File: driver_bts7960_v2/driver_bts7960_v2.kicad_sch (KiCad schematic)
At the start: 28 parts, among them J1 Motor_1, J2 Alimentacion, J6 Motor_2, J7 Conn_02x04_Odd_Even, U1 BTS7960B, U2 BTS7960B, U3 BTS7960B, U4 BTS7960B, U5 74HC244

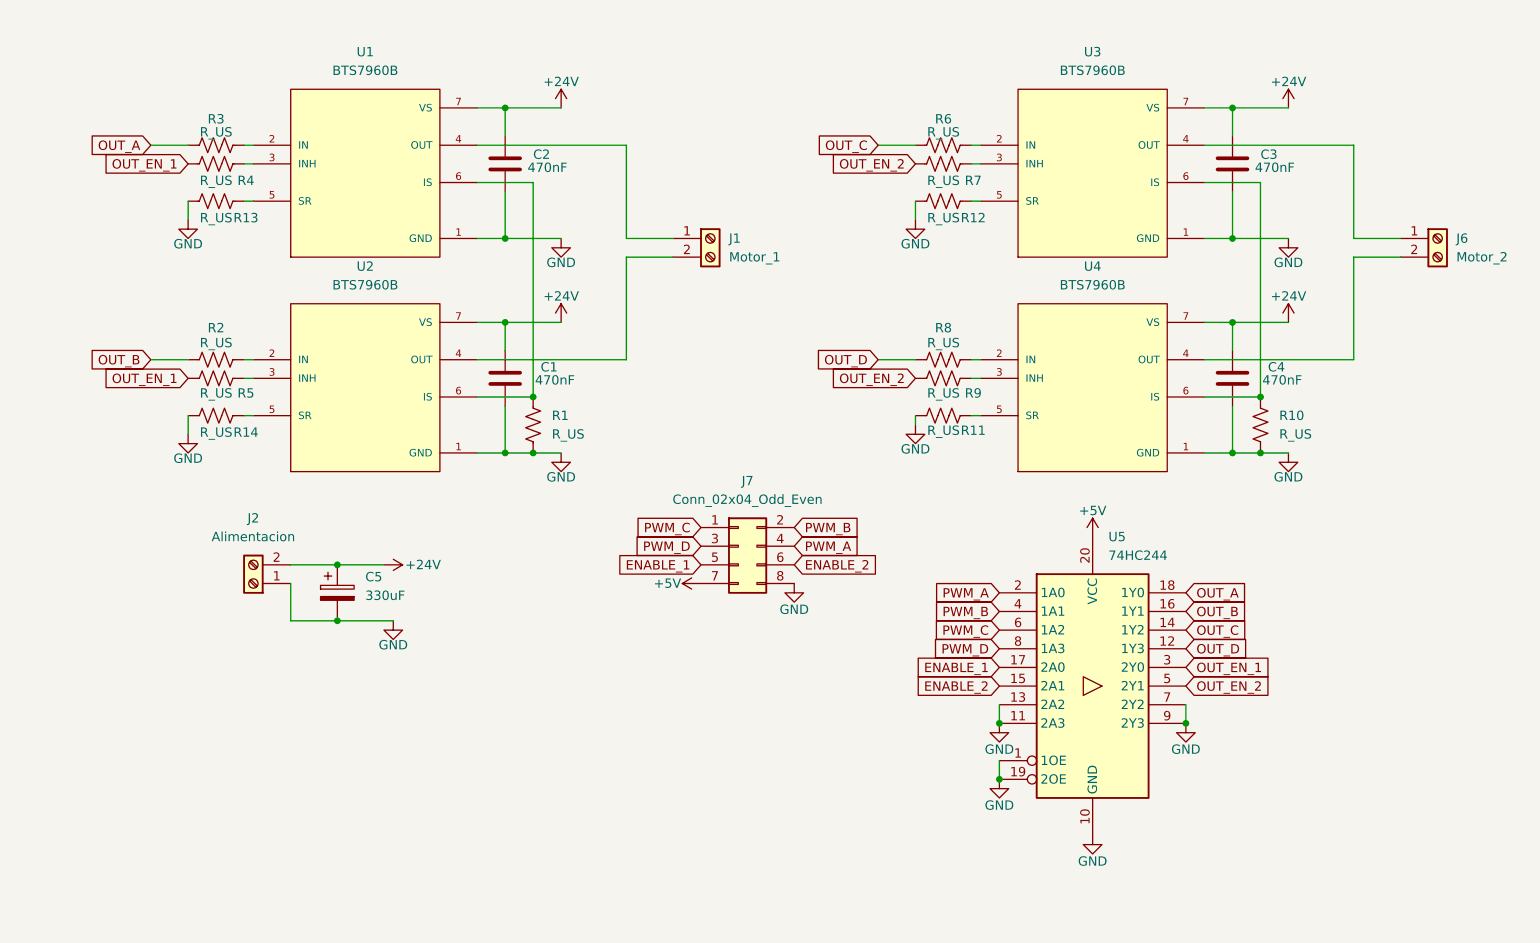
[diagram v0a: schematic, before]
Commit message: .
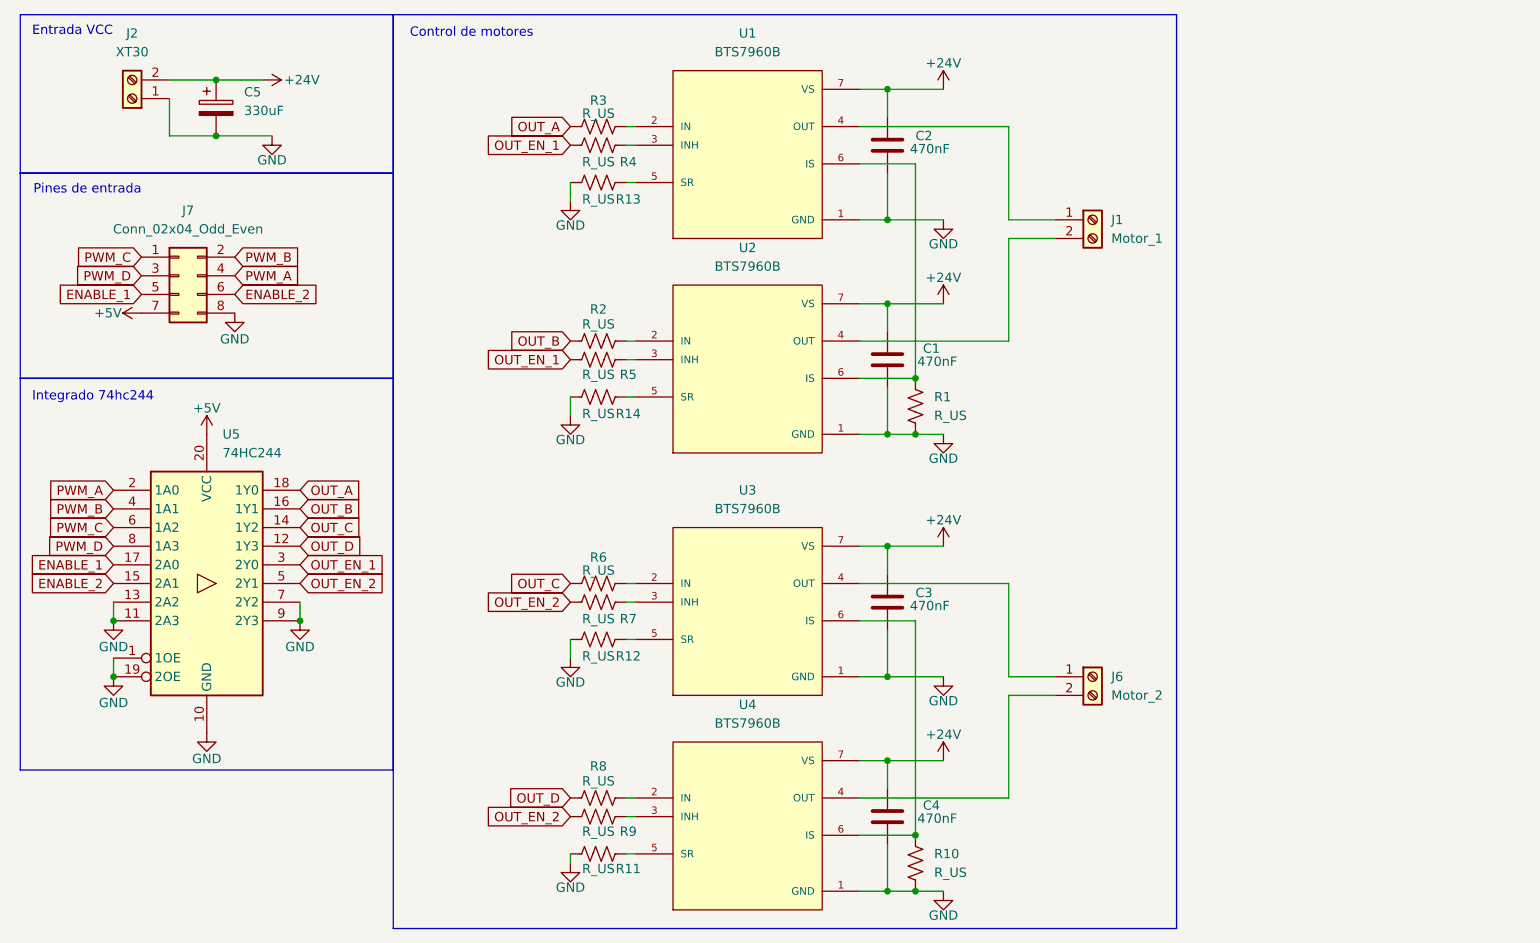
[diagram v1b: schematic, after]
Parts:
- J2: value Alimentacion -> XT30
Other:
- note added: "Control de motores"
- note added: "Entrada VCC"
- note added: "Integrado 74hc244"
- note added: "Pines de entrada"
- moved on the sheet: C1, C2, C3, C4, C5, J1, J2, J6, J7, R1, R10, R11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

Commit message: .
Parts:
- J1, J2, J6: footprint Connector_AMASS:AMASS_XT30UPB-F_1x02_P5.0mm_Vertical -> Connector_AMASS:AMASS_XT30U-F_1x02_P5.0mm_Vertical
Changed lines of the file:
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@@
 			)
 		)
-		(property "Footprint" "Connector_AMASS:AMASS_XT30UPB-F_1x02_P5.0mm_Vertical"
+		(property "Footprint" "Connector_AMASS:AMASS_XT30U-F_1x02_P5.0mm_Vertical"
 			(at 158.75 102.87 0)
 			(hide yes)
@@
 			)
 		)
-		(property "Footprint" "Connector_AMASS:AMASS_XT30UPB-F_1x02_P5.0mm_Vertical"
+		(property "Footprint" "Connector_AMASS:AMASS_XT30U-F_1x02_P5.0mm_Vertical"
 			(at 27.94 24.13 0)
 			(hide yes)
@@
 			)
 		)
-		(property "Footprint" "Connector_AMASS:AMASS_XT30UPB-F_1x02_P5.0mm_Vertical"
+		(property "Footprint" "Connector_AMASS:AMASS_XT30U-F_1x02_P5.0mm_Vertical"
 			(at 158.75 40.64 0)
 			(hide yes)
